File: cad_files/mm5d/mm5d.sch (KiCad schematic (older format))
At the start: 1 part

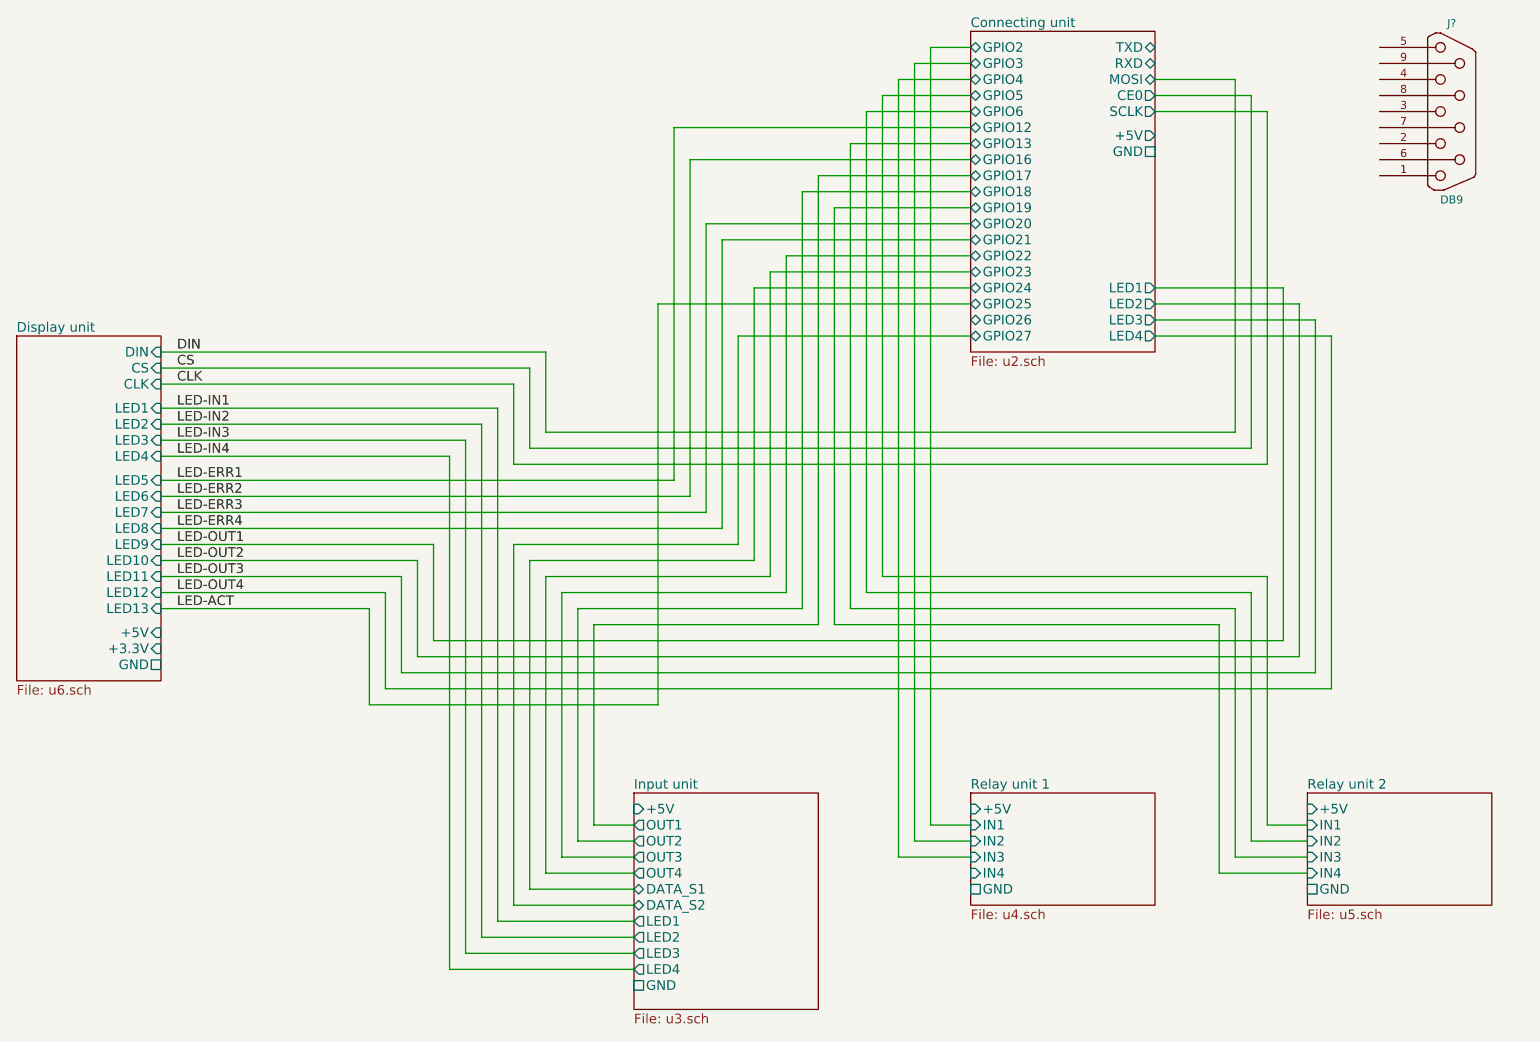
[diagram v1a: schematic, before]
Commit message: 190920
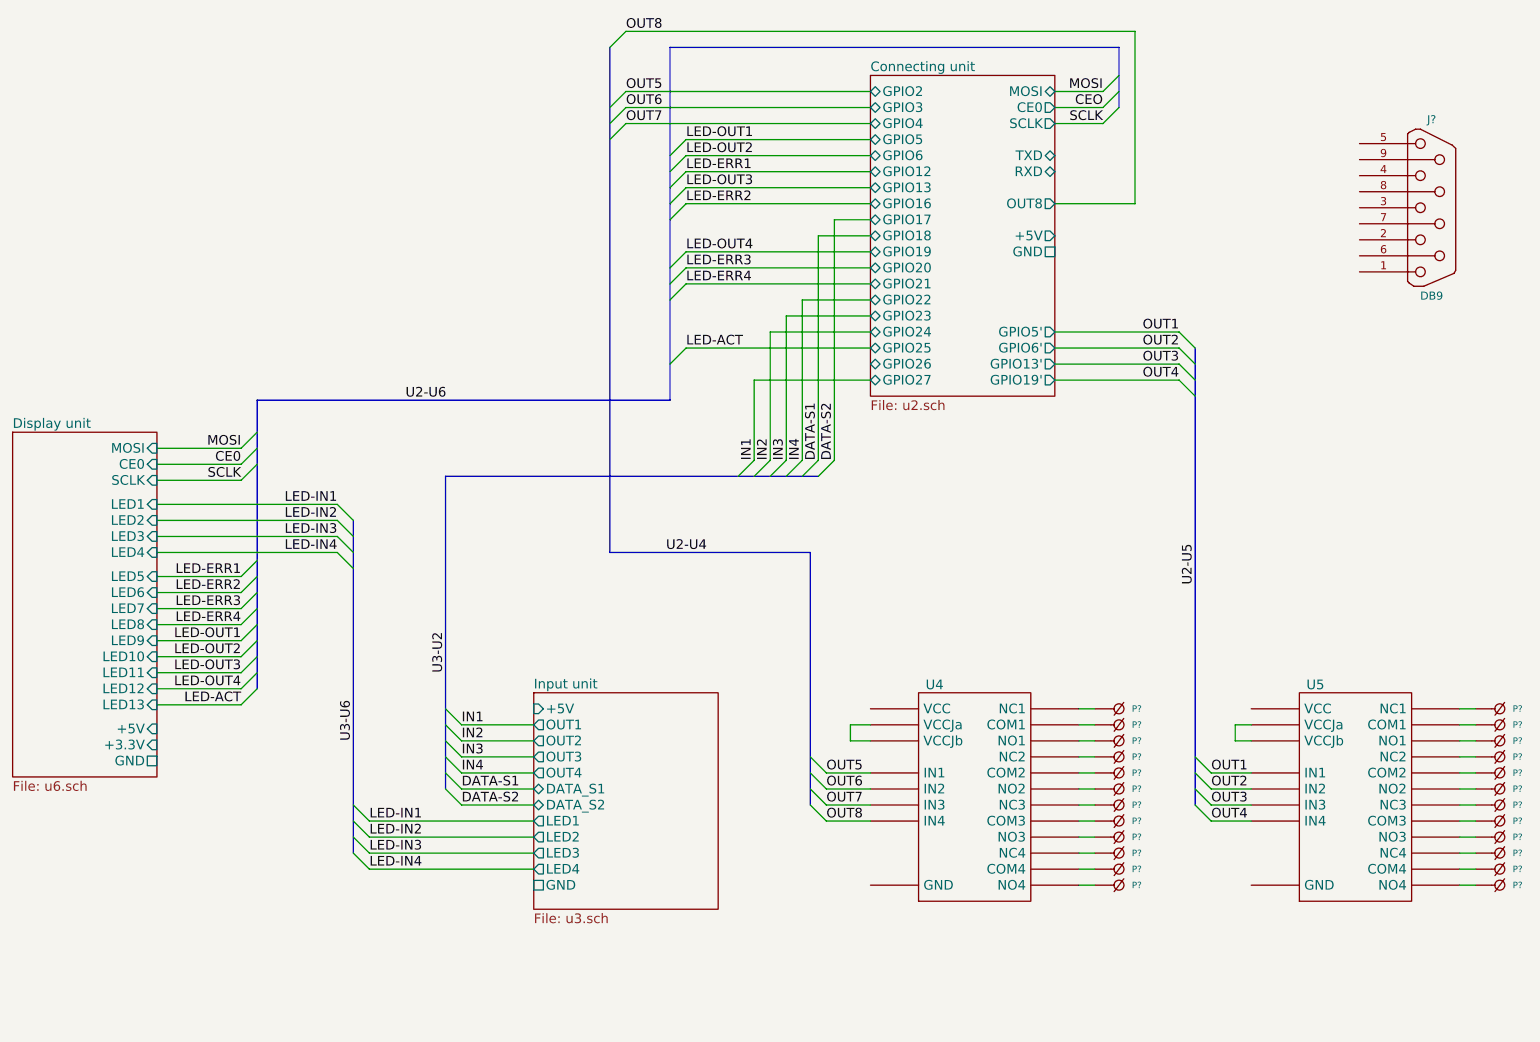
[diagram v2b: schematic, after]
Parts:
- added P? (x24): SCREW_CONN_1, symbol SCREW_CONN_1
- added U4, U5: Relay_panel, symbol Relay_panel
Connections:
- new net: P?.1, U4.~ (VCCJb) (x12)
- new net: P?.1, U5.~ (VCCJb) (x12)
- new net OUT1: U5.~ (VCCJb)
- new net OUT2: U5.~ (VCCJb)
- new net OUT3: U5.~ (VCCJb)
- new net OUT4: U5.~ (VCCJb)
- new net OUT5: U4.~ (VCCJb)
- new net OUT6: U4.~ (VCCJb)
- new net OUT7: U4.~ (VCCJb)
- new net OUT8: U4.~ (VCCJb)
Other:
- moved on the sheet: J?
